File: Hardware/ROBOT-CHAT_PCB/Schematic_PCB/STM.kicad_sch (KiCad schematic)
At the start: 28 parts, among them J2 Conn_02x07_Odd_Even, J3 Conn_01x02, J4 Conn_01x02, SW1 SW_Push_Dual, U1 STM32WB55CEUx, Y1 32MHz

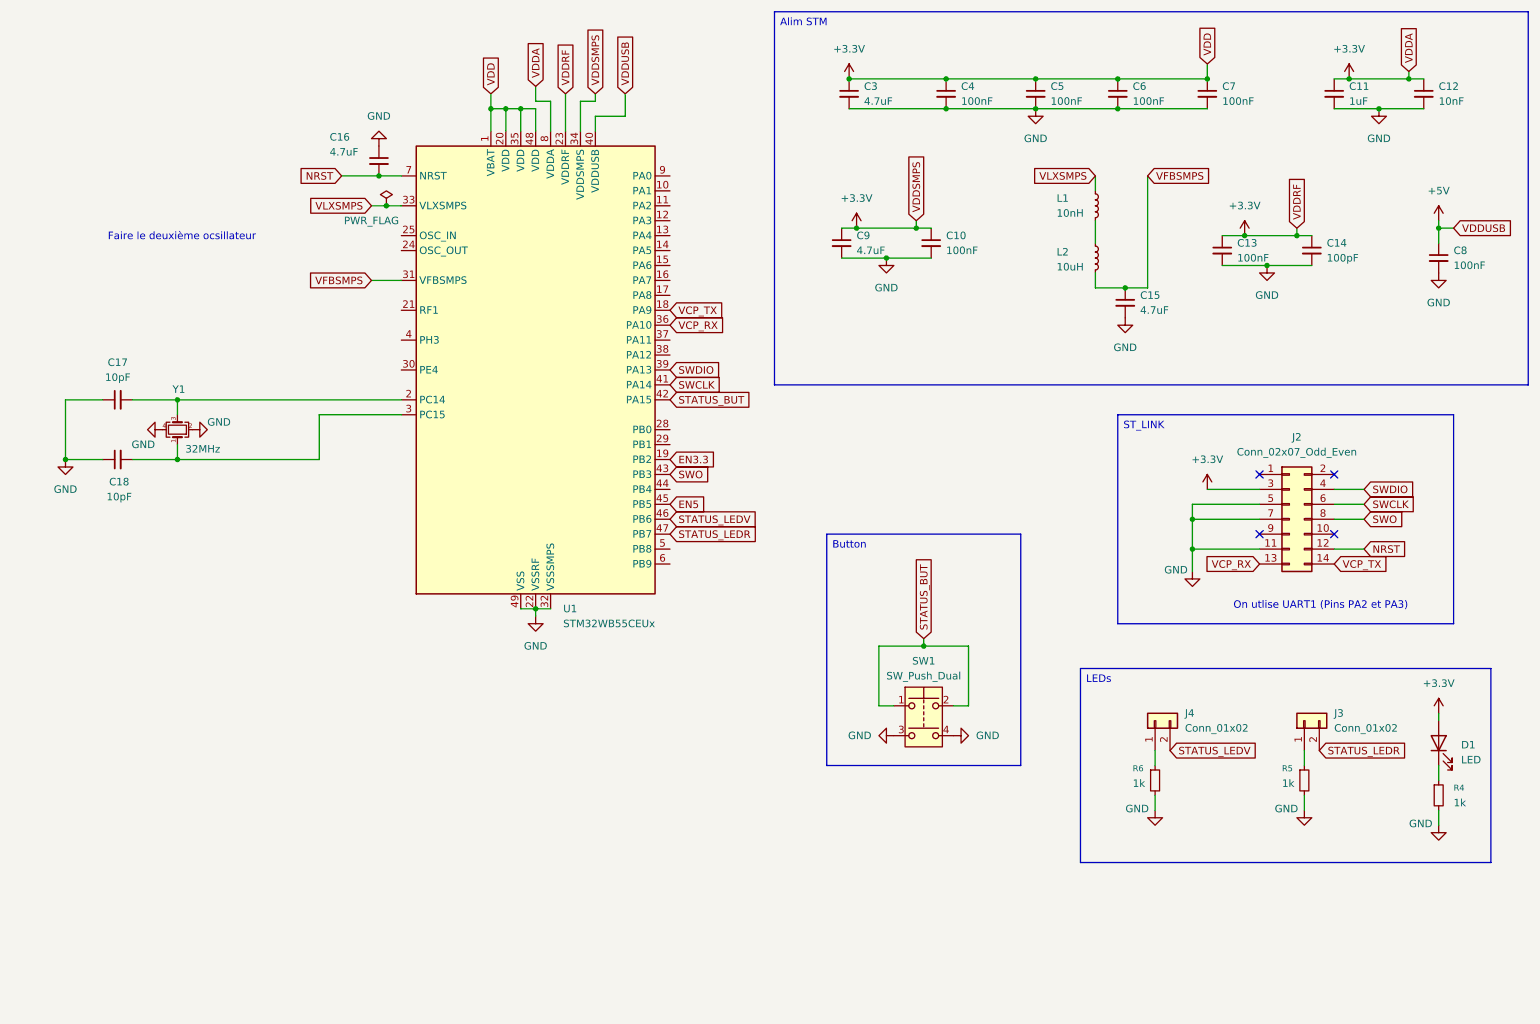
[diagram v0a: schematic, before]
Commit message: Merge PCB v3
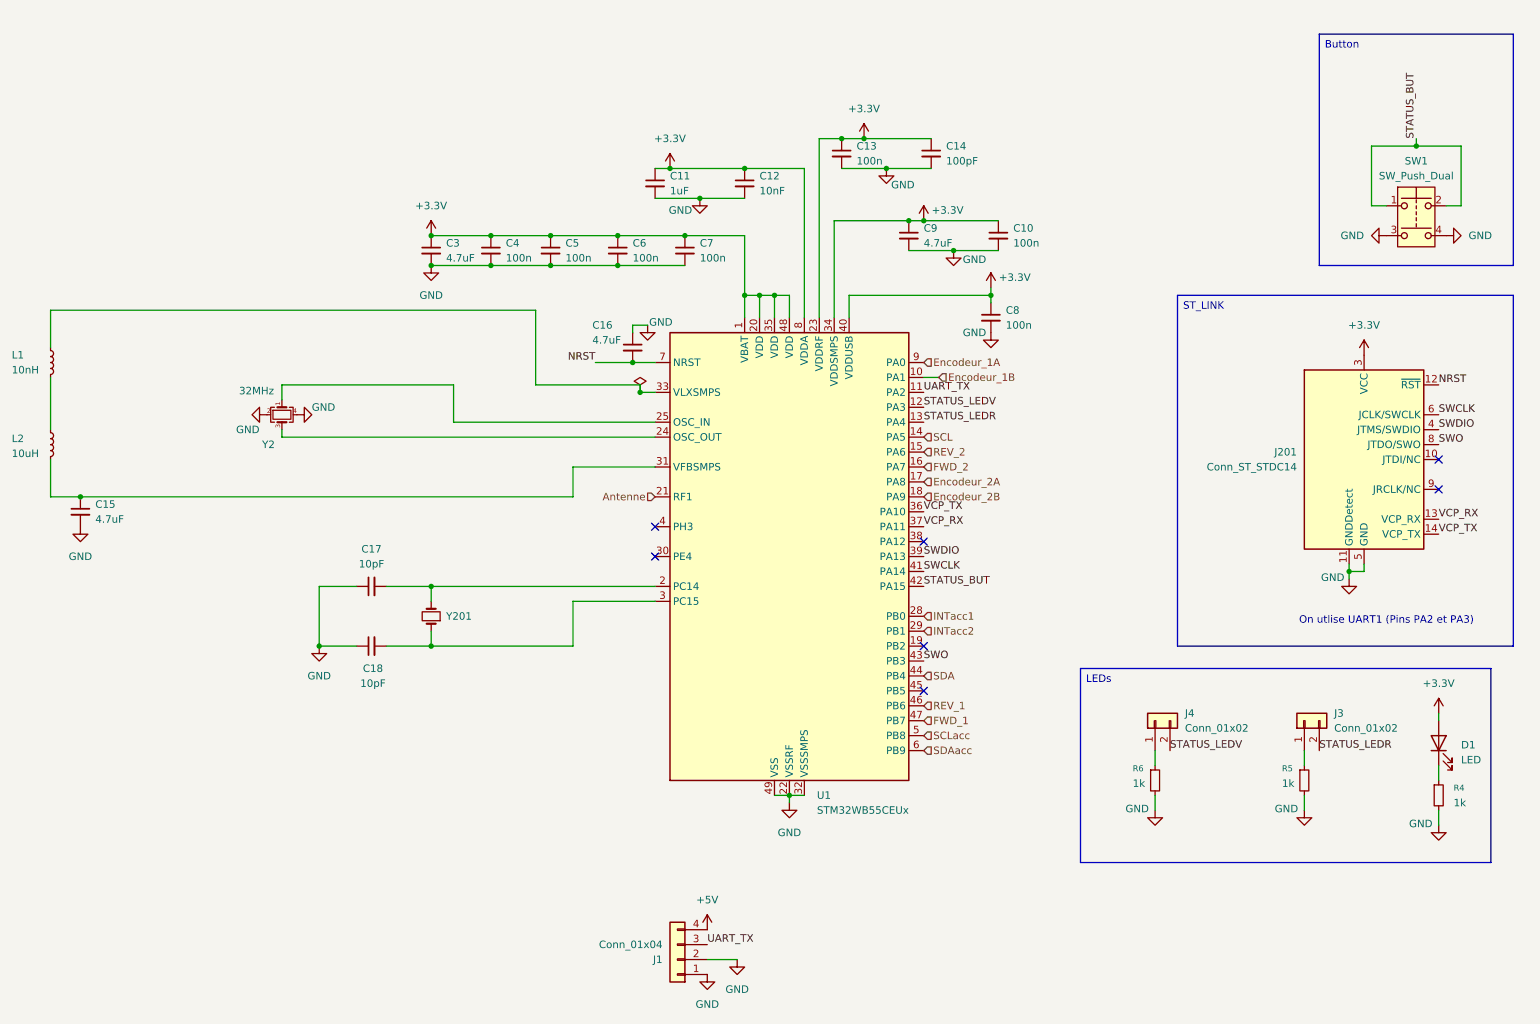
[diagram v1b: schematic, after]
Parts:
- removed J2: Conn_02x07_Odd_Even, symbol Connector_Generic:Conn_02x07_Odd_Even
- removed Y1: 32MHz, XRCGB32M000F2P01R0:XRCGB32M000F2P01R0, symbol Device:Crystal_GND24_Small
- added J1: Conn_01x04, Connector_JST:JST_XH_B4B-XH-AM_1x04_P2.50mm_Vertical, symbol Connector_Generic:Conn_01x04
- added J201: Conn_ST_STDC14, Connector_PinHeader_1.27mm:PinHeader_2x07_P1.27mm_Vertical_SMD, symbol Connector:Conn_ST_STDC14
- added Y2: 32MHz, XRCGB32M000F2P01R0:XRCGB32M000F2P01R0, symbol Device:Crystal_GND24_Small
- added Y201: Crystal_Small, ABS07AIG-32.768KHZ-6-D-T:ABS07AIG-32.768KHZ-6-D-T, symbol Device:Crystal_Small
- C10, C13, C4, C5, C6, C7, C8: value 100nF -> 100n; footprint (none) -> Capacitor_SMD:C_0402_1005Metric
- C11, C15, C16, C3, C9: footprint (none) -> Capacitor_SMD:C_0603_1608Metric
- C12, C14, C17, C18: footprint (none) -> Capacitor_SMD:C_0402_1005Metric
- D1: footprint (none) -> LED_SMD:LED_0603_1608Metric
- J3, J4: footprint (none) -> Connector_JST:JST_PH_B2B-PH-K_1x02_P2.00mm_Vertical
- L1, L2: footprint (none) -> Inductor_SMD:L_0603_1608Metric
- R4, R5, R6: footprint (none) -> Resistor_SMD:R_0402_1005Metric
- SW1: footprint Button_Switch_SMD2:SW_Push_1P1T_NO_6x6mm_H9.5mm -> SW_Push_1P1T_NO_6x6mm_H9.5mm:SW_Push_1P1T_NO_6x6mm_H9.5mm
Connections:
- net +3.3V: now also C8.1, U1.40 (VDDUSB), J201.3 (VCC)
- net +5V: now also J1.4 (Pin_4); no longer C8.1, U1.40 (VDDUSB)
- net GND: now also J1.1 (Pin_1), J1.2 (Pin_2), J201.11 (GNDDetect), J201.5 (GND), J201.7 (GND), Y2.2, Y2.4
- net NRST: now also J201.12 (~{RST})
- net STATUS_LEDR: now also U1.13 (PA4); no longer U1.47 (PB7)
- net STATUS_LEDV: now also U1.12 (PA3); no longer U1.46 (PB6)
- net SWCLK: now also J201.6 (JCLK/SWCLK)
- net SWDIO: now also J201.4 (JTMS/SWDIO)
- net SWO: now also J201.8 (JTDO/SWO)
- net VCP_RX: now also U1.37 (PA11), J201.13 (VCP_RX); no longer U1.36 (PA10)
- net VCP_TX: now also U1.36 (PA10), J201.14 (VCP_TX); no longer U1.18 (PA9)
- net at C18.2, U1.3 (PC15): now also Y201.1
- net at C17.2, U1.2 (PC14): now also Y201.2
- net Encodeur_1B: now reaches U1.10 (PA1)
- net UART_TX: now reaches U1.11 (PA2)
- net UART_TX: now also J1.3 (Pin_3)
- net SCL: now reaches U1.14 (PA5)
- net REV_2: now reaches U1.15 (PA6)
- net FWD_2: now reaches U1.16 (PA7)
- net Encodeur_2A: now reaches U1.17 (PA8)
- net Antenne: now reaches U1.21 (RF1)
- net at U1.24 (OSC_OUT): now also Y2.3
- net at U1.25 (OSC_IN): now also Y2.1
- net INTacc1: now reaches U1.28 (PB0)
- net INTacc2: now reaches U1.29 (PB1)
- net SDA: now reaches U1.44 (PB4)
- net SCLacc: now reaches U1.5 (PB8)
- net SDAacc: now reaches U1.6 (PB9)
- net Encodeur_1A: now reaches U1.9 (PA0)
- net EN3.3: no longer names the net of U1.19 (PB2)
- net EN5: no longer names the net of U1.45 (PB5)
- net VFBSMPS: no longer names the net of C15.1, L2.2, U1.31 (VFBSMPS)
- net VLXSMPS: no longer names the net of L1.1, U1.33 (VLXSMPS)
- new net Encodeur_2B: U1.18 (PA9)
- new net FWD_1: U1.47 (PB7)
- new net REV_1: U1.46 (PB6)
- no-connect marks 4 -> 7
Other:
- note removed: "Faire le deuxième ocsillateur"
- moved on the sheet: C10, C11, C12, C13, C14, C15, C16, C17, C18, C3, C4, C5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
